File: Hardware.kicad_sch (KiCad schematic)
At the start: 29 parts, among them J1 Conn_01x06_Socket, J5 Conn_01x05_Socket, Q1 BC849, Q2 BC849, SW1 Push_Button, SW2 Push_Button, U1 ESP32-WROOM-32, U9 AMS1117-3.3

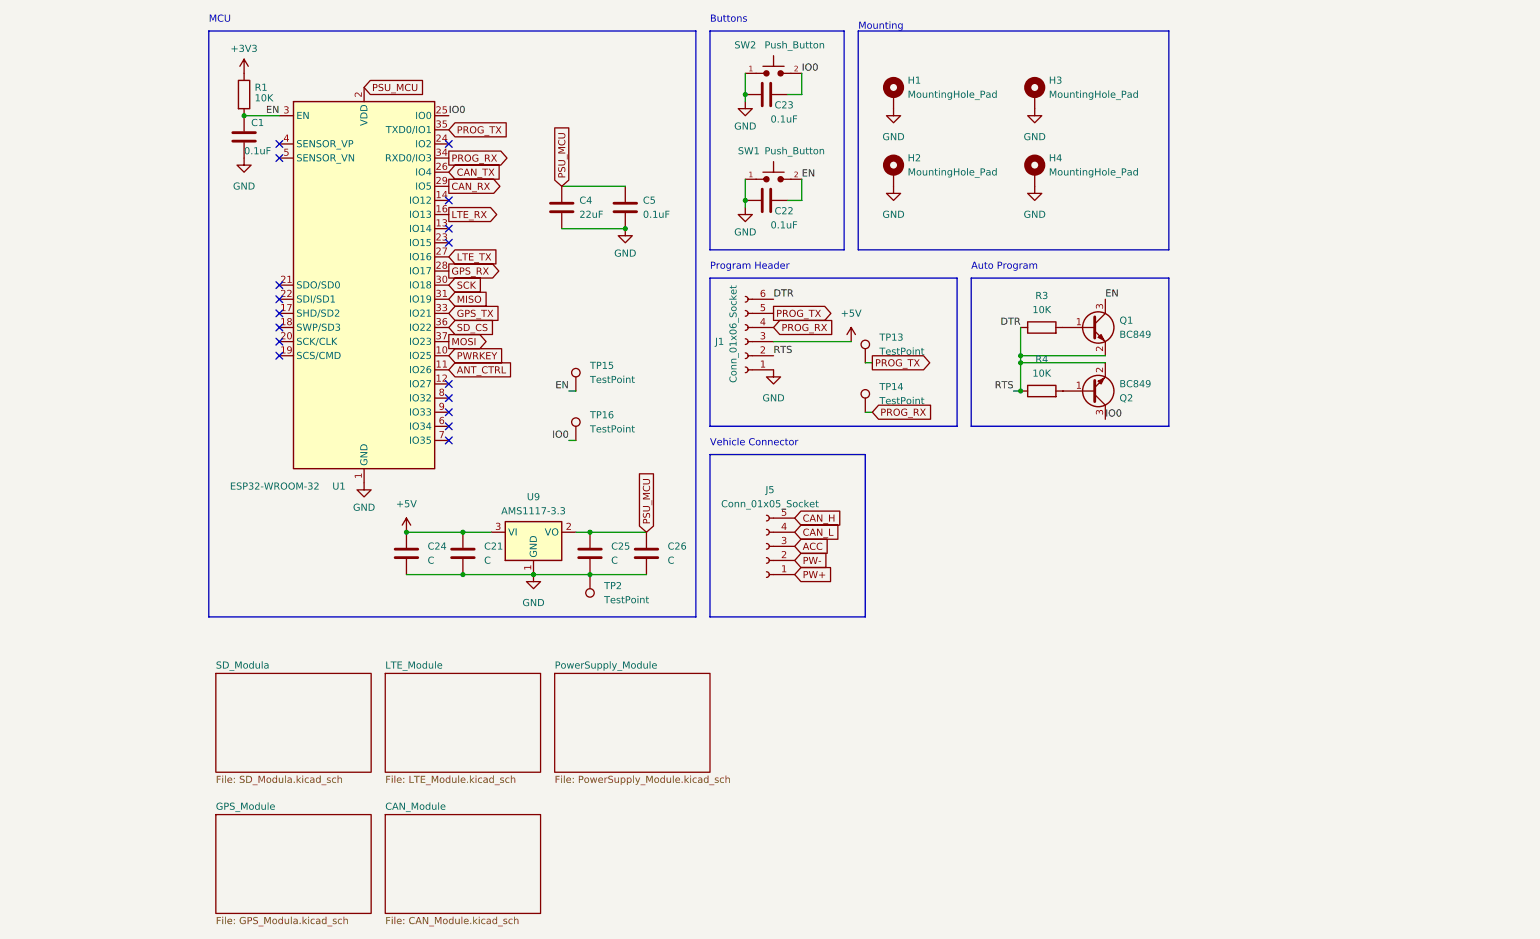
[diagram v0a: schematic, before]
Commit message: done most of the schematics
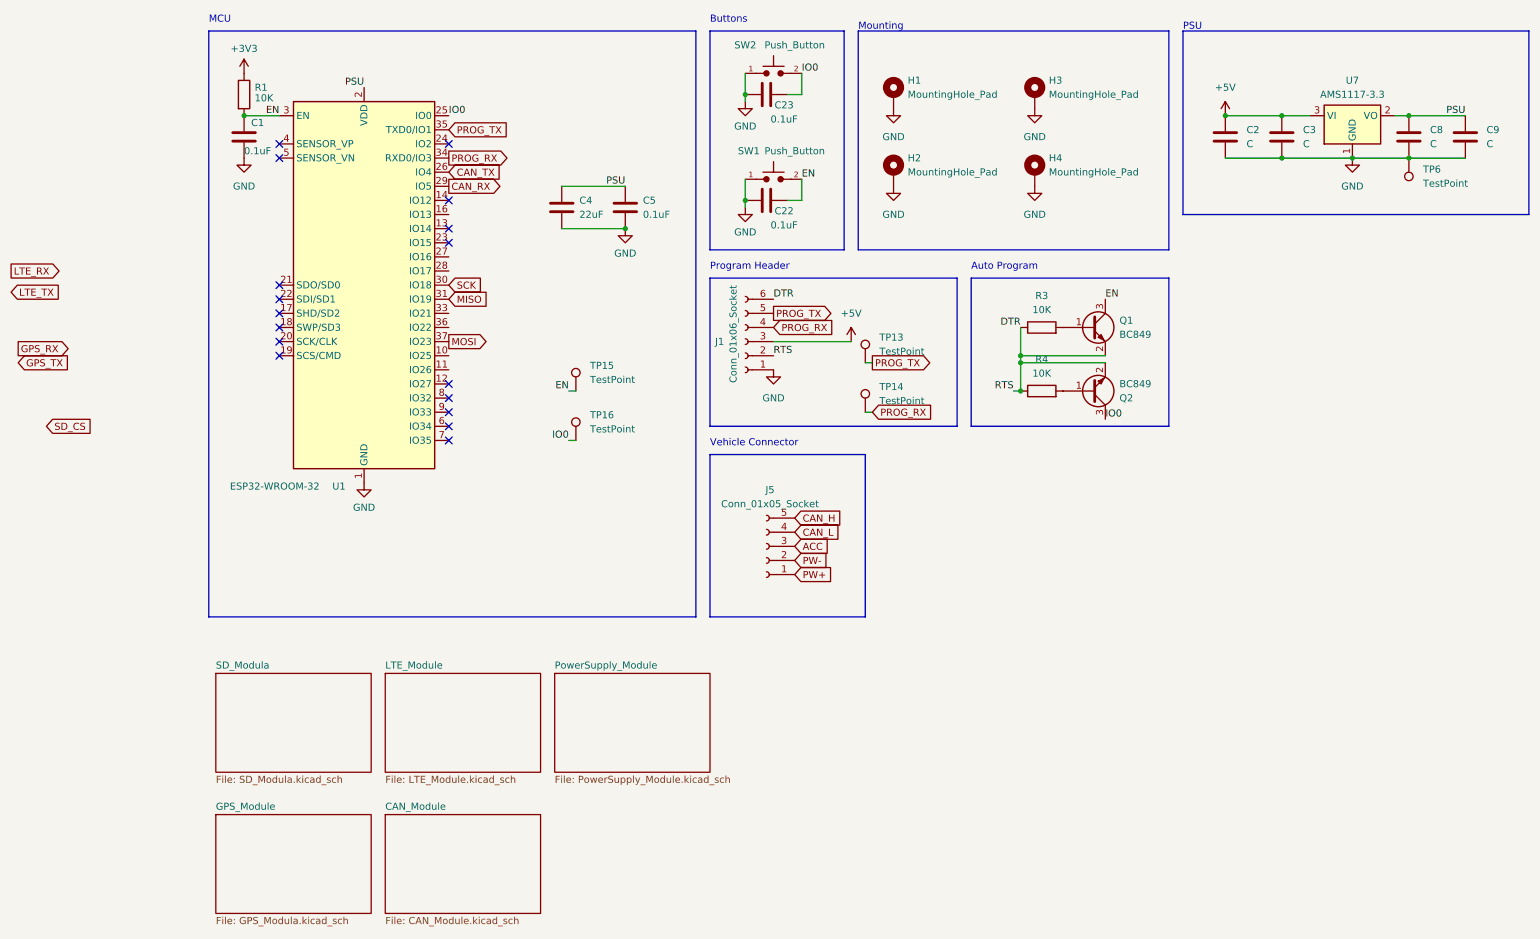
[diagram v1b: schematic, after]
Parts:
- removed C21, C24, C25, C26: C, symbol Device:C
- removed TP2: TestPoint, symbol Connector:TestPoint
- removed U9: AMS1117-3.3, Package_TO_SOT_SMD:SOT-223-3_TabPin2, symbol Regulator_Linear:AMS1117-3.3
- added C2, C3, C8, C9: C, symbol Device:C
- added TP6: TestPoint, symbol Connector:TestPoint
- added U7: AMS1117-3.3, Package_TO_SOT_SMD:SOT-223-3_TabPin2, symbol Regulator_Linear:AMS1117-3.3
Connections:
- net +5V: now also C2.1, C3.1, U7.3 (VI)
- net GND: now also C2.2, C3.2, C8.2, C9.2, TP6.1, U7.1 (GND)
- net GPS_RX: no longer U1.28 (IO17)
- net GPS_TX: no longer U1.33 (IO21)
- net LTE_RX: no longer U1.16 (IO13)
- net LTE_TX: no longer U1.27 (IO16)
- net SD_CS: no longer U1.36 (IO22)
- net ANT_CTRL: no longer names the net of U1.11 (IO26)
- net PSU_MCU renamed PSU
- net PSU: now also C8.1, C9.1, U7.2 (VO)
- net PWRKEY: no longer names the net of U1.10 (IO25)
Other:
- note added: "PSU"

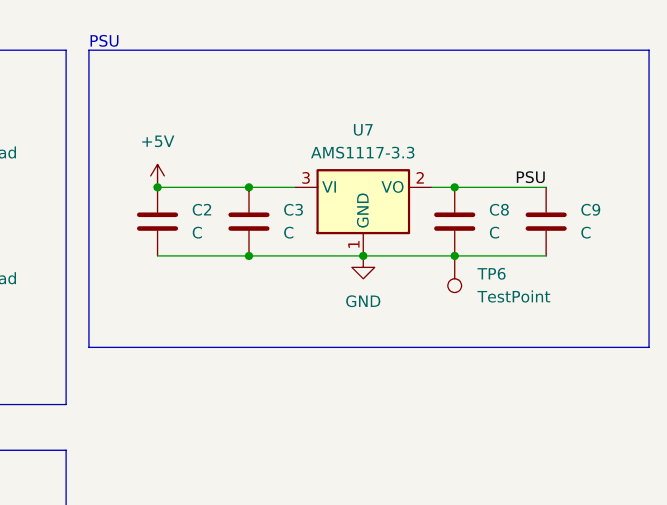
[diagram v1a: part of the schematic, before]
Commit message: done refacoring
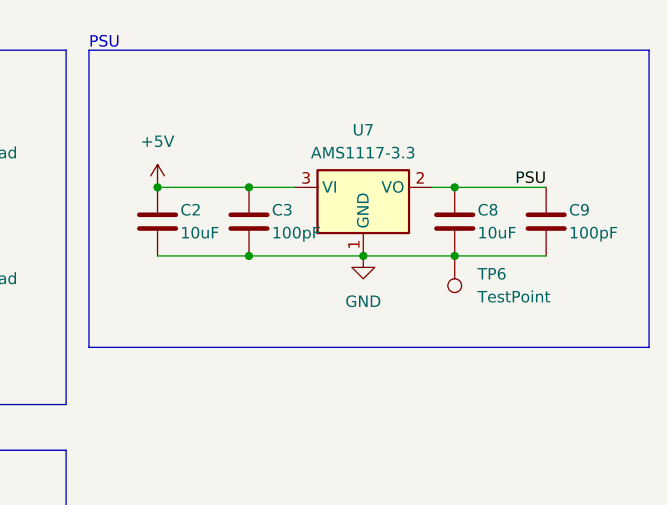
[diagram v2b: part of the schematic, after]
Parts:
- C2, C8: value C -> 10uF
- C3, C9: value C -> 100pF
- H1, H2, H3, H4: footprint (none) -> MountingHole:MountingHole_3.2mm_M3_DIN965_Pad
- J5: footprint (none) -> Connector_PinHeader_1.00mm:PinHeader_1x05_P1.00mm_Vertical
- R1, R3, R4: footprint Resistor_SMD:R_1206_3216Metric_Pad1.30x1.75mm_HandSolder -> (none)
- TP13, TP14, TP15, TP16, TP6: footprint (none) -> TestPoint:TestPoint_Pad_D2.5mm
